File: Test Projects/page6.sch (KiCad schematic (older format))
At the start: 100 parts, among them P22 CONN_01X08, P23 CONN_01X08, P24 CONN_01X08, P25 CONN_01X08, P26 CONN_01X08, P27 CONN_01X08, P28 CONN_01X08, P29 CONN_01X08, P74 CONN_01X08, P75 CONN_01X08, P76 CONN_01X08, P77 CONN_01X08, P78 CONN_01X08, P79 CONN_01X08, P80 CONN_01X08, P81 CONN_01X08, P87 CONN_01X01, P88 CONN_01X01, U23 SF-74HC595, U24 SF-74HC595, U25 SF-74HC595, U26 SF-74HC595, U27 SF-74HC595, U28 SF-74HC595, U29 SF-74HC595, U30 SF-74HC595

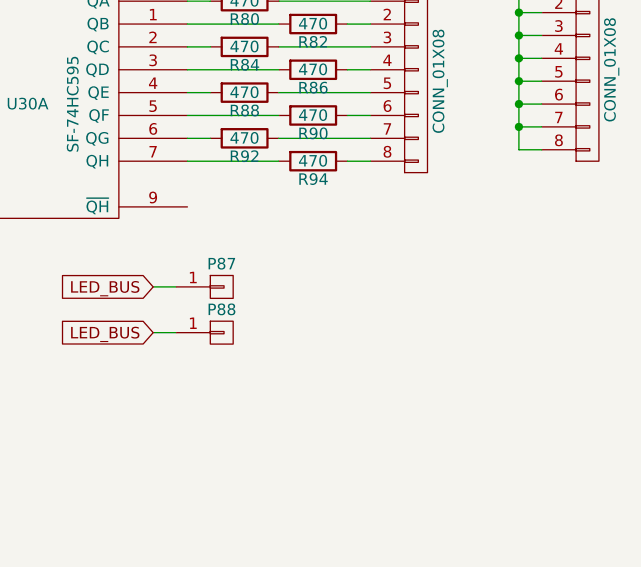
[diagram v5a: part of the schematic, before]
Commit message: went to production
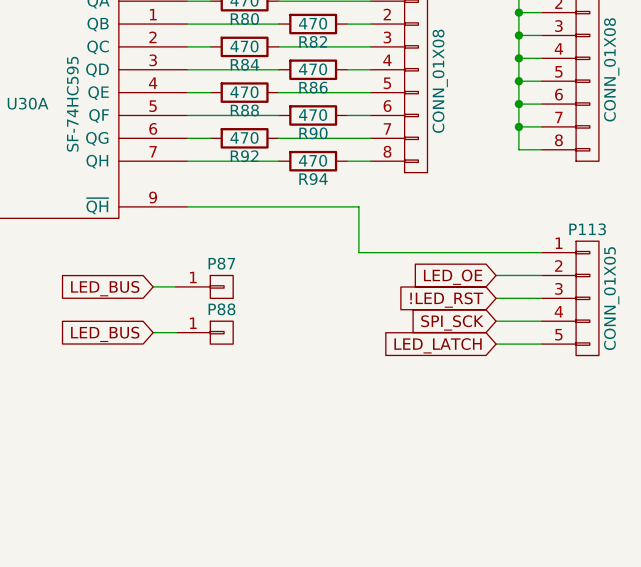
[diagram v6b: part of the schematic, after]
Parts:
- added P113: CONN_01X05, Pin_Headers:Pin_Header_Straight_1x05, symbol CONN_01X05
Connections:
- net !LED_RST: now also P113.3 (P3)
- net LED_LATCH: now also P113.5 (P5)
- net LED_OE: now also P113.2 (P2)
- net SPI_SCK: now also P113.4 (P4)
- net at U30.9 (~QH): now also P113.1 (P1)
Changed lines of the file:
@@
 $EndComp
 $Comp
-L +5V #PWR0111
+L +5V #PWR0112
 U 1 1 568A1F71
 P 1000 6150
-F 0 "#PWR0111" H 1000 6000 50  0001 C CNN
+F 0 "#PWR0112" H 1000 6000 50  0001 C CNN
 F 1 "+5V" H 1000 6290 50  0000 C CNN
 F 2 "" H 1000 6150 50  0000 C CNN
@@
 	6650 4700 6650 4950
 $Comp
-L GND #PWR0112
+L GND #PWR0113
 U 1 1 568A29A6
 P 1000 7450
-F 0 "#PWR0112" H 1000 7200 50  0001 C CNN
+F 0 "#PWR0113" H 1000 7200 50  0001 C CNN
 F 1 "GND" H 1000 7300 50  0000 C CNN
 F 2 "" H 1000 7450 50  0000 C CNN
@@
 $EndComp
 $Comp
-L GND #PWR0113
+L GND #PWR0114
 U 1 1 568A2A18
 P 1800 7450
-F 0 "#PWR0113" H 1800 7200 50  0001 C CNN
+F 0 "#PWR0114" H 1800 7200 50  0001 C CNN
 F 1 "GND" H 1800 7300 50  0000 C CNN
 F 2 "" H 1800 7450 50  0000 C CNN
@@
 $EndComp
 $Comp
-L GND #PWR0114
+L GND #PWR0115
 U 1 1 568A2A83
 P 2600 7450
-F 0 "#PWR0114" H 2600 7200 50  0001 C CNN
+F 0 "#PWR0115" H 2600 7200 50  0001 C CNN
 F 1 "GND" H 2600 7300 50  0000 C CNN
 F 2 "" H 2600 7450 50  0000 C CNN
@@
 $EndComp
 $Comp
-L GND #PWR0115
+L GND #PWR0116
 U 1 1 568A2A89
 P 3400 7450
-F 0 "#PWR0115" H 3400 7200 50  0001 C CNN
+F 0 "#PWR0116" H 3400 7200 50  0001 C CNN
 F 1 "GND" H 3400 7300 50  0000 C CNN
 F 2 "" H 3400 7450 50  0000 C CNN
@@
 $EndComp
 $Comp
-L GND #PWR0116
+L GND #PWR0117
 U 1 1 568A2B8F
 P 4200 7450
-F 0 "#PWR0116" H 4200 7200 50  0001 C CNN
+F 0 "#PWR0117" H 4200 7200 50  0001 C CNN
 F 1 "GND" H 4200 7300 50  0000 C CNN
 F 2 "" H 4200 7450 50  0000 C CNN
@@
 $EndComp
 $Comp
-L GND #PWR0117
+L GND #PWR0118
 U 1 1 568A2B95
 P 5000 7450
-F 0 "#PWR0117" H 5000 7200 50  0001 C CNN
+F 0 "#PWR0118" H 5000 7200 50  0001 C CNN
 F 1 "GND" H 5000 7300 50  0000 C CNN
 F 2 "" H 5000 7450 50  0000 C CNN
@@
 $EndComp
 $Comp
-L GND #PWR0118
+L GND #PWR0119
 U 1 1 568A2B9B
 P 5800 7450
-F 0 "#PWR0118" H 5800 7200 50  0001 C CNN
+F 0 "#PWR0119" H 5800 7200 50  0001 C CNN
 F 1 "GND" H 5800 7300 50  0000 C CNN
 F 2 "" H 5800 7450 50  0000 C CNN
@@
 $EndComp
 $Comp
-L GND #PWR0119
+L GND #PWR0120
 U 1 1 568A2BA1
 P 6600 7450
-F 0 "#PWR0119" H 6600 7200 50  0001 C CNN
+F 0 "#PWR0120" H 6600 7200 50  0001 C CNN
 F 1 "GND" H 6600 7300 50  0000 C CNN
 F 2 "" H 6600 7450 50  0000 C CNN
@@
 $EndComp
 $Comp
-L +5V #PWR0120
+L +5V #PWR0121
 U 1 1 568A2BE7
 P 1800 6150
-F 0 "#PWR0120" H 1800 6000 50  0001 C CNN
+F 0 "#PWR0121" H 1800 6000 50  0001 C CNN
 F 1 "+5V" H 1800 6290 50  0000 C CNN
 F 2 "" H 1800 6150 50  0000 C CNN
@@
 $EndComp
 $Comp
-L +5V #PWR0121
+L +5V #PWR0122
 U 1 1 568A2C52
 P 2600 6150
-F 0 "#PWR0121" H 2600 6000 50  0001 C CNN
+F 0 "#PWR0122" H 2600 6000 50  0001 C CNN
 F 1 "+5V" H 2600 6290 50  0000 C CNN
 F 2 "" H 2600 6150 50  0000 C CNN
@@
 $EndComp
 $Comp
-L +5V #PWR0122
+L +5V #PWR0123
 U 1 1 568A2CBD
 P 3400 6150
-F 0 "#PWR0122" H 3400 6000 50  0001 C CNN
+F 0 "#PWR0123" H 3400 6000 50  0001 C CNN
 F 1 "+5V" H 3400 6290 50  0000 C CNN
 F 2 "" H 3400 6150 50  0000 C CNN
@@
 $EndComp
 $Comp
-L +5V #PWR0123
+L +5V #PWR0124
 U 1 1 568A2D28
 P 4200 6150
-F 0 "#PWR0123" H 4200 6000 50  0001 C CNN
+F 0 "#PWR0124" H 4200 6000 50  0001 C CNN
 F 1 "+5V" H 4200 6290 50  0000 C CNN
 F 2 "" H 4200 6150 50  0000 C CNN
@@
 $EndComp
 $Comp
-L +5V #PWR0124
+L +5V #PWR0125
 U 1 1 568A2D93
 P 5000 6150
-F 0 "#PWR0124" H 5000 6000 50  0001 C CNN
+F 0 "#PWR0125" H 5000 6000 50  0001 C CNN
 F 1 "+5V" H 5000 6290 50  0000 C CNN
 F 2 "" H 5000 6150 50  0000 C CNN
@@
 $EndComp
 $Comp
-L +5V #PWR0125
+L +5V #PWR0126
 U 1 1 568A2DFE
 P 5800 6150
-F 0 "#PWR0125" H 5800 6000 50  0001 C CNN
+F 0 "#PWR0126" H 5800 6000 50  0001 C CNN
 F 1 "+5V" H 5800 6290 50  0000 C CNN
 F 2 "" H 5800 6150 50  0000 C CNN
@@
 $EndComp
 $Comp
-L +5V #PWR0126
+L +5V #PWR0127
 U 1 1 568A2E69
 P 6600 6150
-F 0 "#PWR0126" H 6600 6000 50  0001 C CNN
+F 0 "#PWR0127" H 6600 6000 50  0001 C CNN
 F 1 "+5V" H 6600 6290 50  0000 C CNN
 F 2 "" H 6600 6150 50  0000 C CNN
@@
 	7750 3300 1600 3300
 $Comp
-L +5V #PWR0127
+L +5V #PWR0128
 U 1 1 56A369B9
 P 1350 3250
-F 0 "#PWR0127" H 1350 3100 50  0001 C CNN
+F 0 "#PWR0128" H 1350 3100 50  0001 C CNN
 F 1 "+5V" H 1350 3390 50  0000 C CNN
 F 2 "" H 1350 3250 50  0000 C CNN
@@
 Connection ~ 1200 4050
 $Comp
-L GND #PWR0128
+L GND #PWR0129
 U 1 1 56A37981
 P 1200 4800
-F 0 "#PWR0128" H 1200 4550 50  0001 C CNN
+F 0 "#PWR0129" H 1200 4550 50  0001 C CNN
 F 1 "GND" H 1200 4650 50  0000 C CNN
 F 2 "" H 1200 4800 50  0000 C CNN
@@
 Text GLabel 7900 6300 0    50   Input ~ 0
 LED_BUS
+$Comp
+L CONN_01X05 P113
+U 1 1 56B72D95
+P 9800 6150
+F 0 "P113" H 9800 6450 50  0000 C CNN
+F 1 "CONN_01X05" V 9900 6150 50  0000 C CNN
+F 2 "Pin_Headers:Pin_Header_Straight_1x05" H 9800 6150 50  0001 C CNN
+F 3 "" H 9800 6150 50  0000 C CNN
+	1    9800 6150
+	1    0    0    -1
+$EndComp
+Text GLabel 9400 6350 0    50   Input ~ 0
+LED_LATCH
+Text GLabel 9400 6250 0    50   Input ~ 0
+SPI_SCK
+Text GLabel 9400 6150 0    50   Input ~ 0
+!LED_RST
+Text GLabel 9400 6050 0    50   Input ~ 0
+LED_OE
+Wire Wire Line
+	8050 5750 8800 5750
+Wire Wire Line
+	8800 5750 8800 5950
+Wire Wire Line
+	8800 5950 9600 5950
+Wire Wire Line
+	9400 6050 9600 6050
+Wire Wire Line
+	9400 6150 9600 6150
+Wire Wire Line
+	9400 6250 9600 6250
+Wire Wire Line
+	9400 6350 9600 6350
 $EndSCHEMATC
